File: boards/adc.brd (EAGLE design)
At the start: 49.6 x 25.6 mm, 42 parts, among them U1 ADS1194CPAG

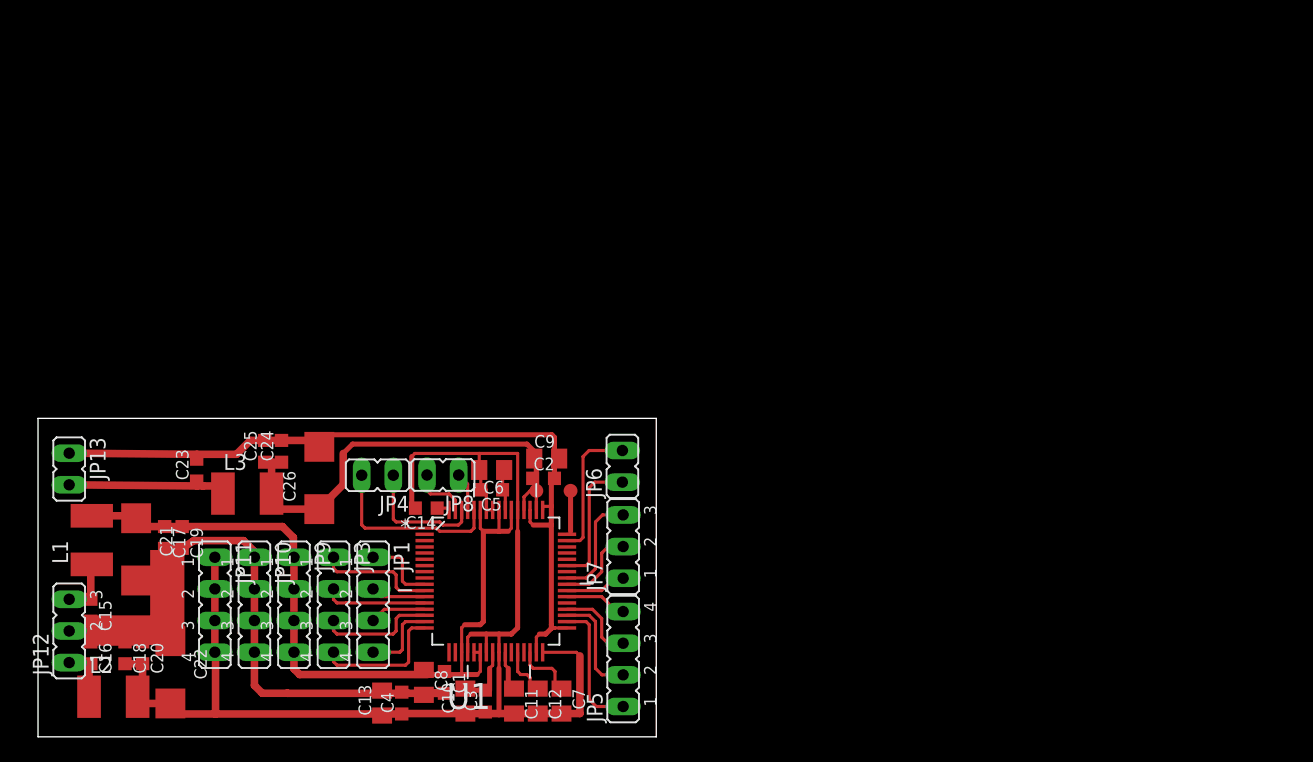
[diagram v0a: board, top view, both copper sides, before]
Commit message: put all the downloaded files into directories
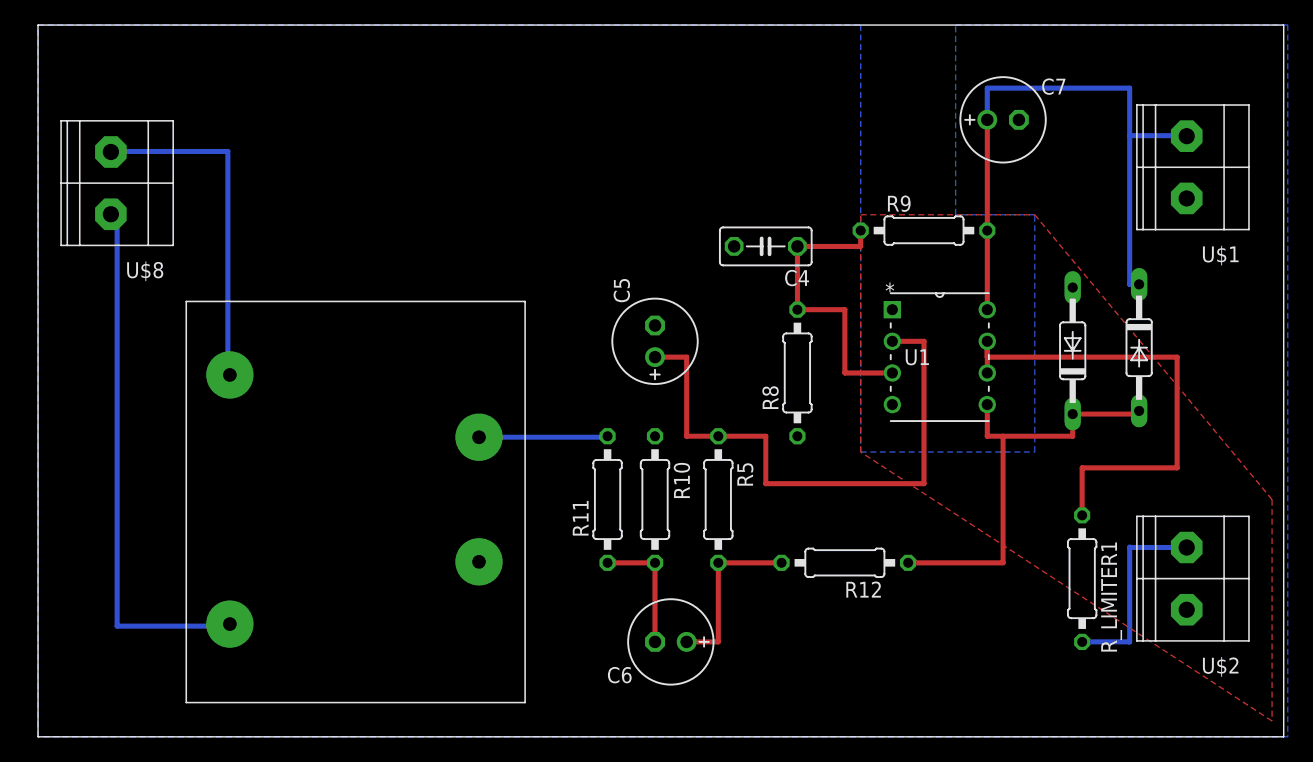
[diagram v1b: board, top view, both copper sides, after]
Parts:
- removed C1, C15, C16, C19, C2, C20, C23, C25, C3: 100n, rcl:C0603K
- removed C10, C12: 10u, rcl:C0805K
- removed C11, C13, C8, C9: 1u, rcl:C0805K
- removed C14, C17, C18, C24: 100p, rcl:C0603K
- removed C21, C22, C26: 47u, rcl:SMC_C
- removed JP1: AINneg, jumper:JP4
- removed JP10: AINgnd, jumper:JP4
- removed JP11: AINvss, jumper:JP4
- removed JP12: PWR1, jumper:JP2
- removed JP13: PWR2, jumper:JP1
- removed JP3: AINpos, jumper:JP4
- removed JP4: RL2, jumper:JP1
- removed JP5: CTRL2, jumper:JP4
- removed JP6: CTRL1, jumper:JP1
- removed JP7: CTRL2, jumper:JP2
- removed JP8: RL1, jumper:JP1
- removed JP9: AINvdd, jumper:JP4
- removed L1, L2, L3: 22u, rcl:L1812
- added R10, R11, R12, R5, R8, R9, R_LIMITER1: (no value), ee2parts:0207/10
- added U$1, U$2, U$8: CTB1500/2, eko-parts:CTB1500-2
- added U$5: (no value), Pauls_parts:4408
- added U$6, U$7: SD103A, Pauls_parts:D035-10
- C4: value 100n -> (none); device rcl:C0603K -> ee2parts:C050-030-075
- C5: value 100n -> (none); device rcl:C0603K -> ee2parts:E2,5-7---100UF
- C6, C7: value 1u -> (none); device rcl:C0805K -> ee2parts:E2,5-7---100UF
- U1: value ADS1194CPAG -> MCP602-E/P; device adc-ti:QFP50P1200X1200X120-64N -> MCP:DIP254P762X508-8P
- moved C7 58.6 mm to (77.5, 49.5), turned to 0 degrees
- moved C4 46.9 mm to (58.4, 39.4), turned to 180 degrees
- moved U1 41.9 mm to (76.2, 26.7)
- moved C6 19.9 mm to (50.8, 7.62)
- moved C5 17.7 mm to (49.5, 31.8), turned to 90 degrees
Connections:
- removed net +2V5: C1.1, C17.1, C19.1, C21.+, C8.1, JP9.1, JP9.2, JP9.3, JP9.4, L1.2, U1.19, U1.21, U1.22, U1.54, U1.56, U1.59
- removed net +2V5/1: C15.1, JP12.3, L1.1
- removed net +3V3: C2.1, C24.1, C25.1, C26.+, C9.1, L3.2, U1.48, U1.50, U1.52
- removed net +3V3/1: C23.1, JP13.2, L3.1
- removed net -2V5: C10.1, C11.2, C12.2, C13.1, C14.2, C18.2, C20.2, C22.-, C3.1, C4.1, C5.2, C6.2, C7.2, JP11.1, JP11.2, JP11.3, JP11.4, L2.2, U1.20, U1.23, U1.25, U1.32, U1.53, U1.57, U1.58
- removed net -2V5/1: C16.2, JP12.1, L2.1
- removed net AGND: C1.2, C13.2, C15.2, C16.1, C17.2, C18.1, C19.2, C20.1, C21.-, C22.+, C4.2, C8.2, JP10.1, JP10.2, JP10.3, JP10.4, JP12.2
- removed net DAISY_IN: JP7.3, U1.41
- removed net DIN: JP5.1, U1.34
- removed net DOUT: JP6.1, U1.43
- removed net N$11: JP3.1, U1.10
- removed net N$13: JP3.3, U1.14
- removed net N$14: JP3.2, U1.12
- removed net N$15: JP4.1, U1.62
- removed net N$16: JP4.2, U1.60
- removed net N$24: JP8.2, U1.63
- removed net N$3: C7.1, U1.30
- removed net N$4: C12.1, U1.28
- removed net N$5: C11.1, U1.26
- removed net N$6: JP1.4, U1.15
- removed net N$7: C14.1, U1.64
- removed net N$8: JP1.3, U1.13
- removed net N$9: JP1.2, U1.11
- removed net SCLK: JP7.2, U1.40
- removed net START: JP5.4, U1.38
- removed net ~CS: JP7.1, U1.39
- removed net ~DRDY: JP6.2, U1.47
- removed net ~PWDN: JP5.2, U1.35
- removed net ~RESET: JP5.3, U1.36
- new net N$18: R11.2, U$5.PIN7
- new net N$21: C6.+, R12.2, R5.2
- new net V+: C7.+, R9.2, U$1.P$2, U$6.C, U1.8
- new net V_IN1: U$5.PIN5, U$8.P$2
- new net V_IN2: U$5.PIN1, U$8.P$1
- new net V_OUT: R_LIMITER1.2, U$2.P$2
- net GND: now also C4.2, C5.-, C7.-, R10.1, R8.1, U$2.P$1, U$5.PIN9, U$7.A, U1.4; no longer C2.2, C23.2, C24.2, C25.2, C26.-, C9.2, JP13.1, U1.31, U1.33, U1.49, U1.51
- net N$1: now also R_LIMITER1.1, U1.6, U1.7; no longer C10.2, C3.2, U1.24
- net N$10: now also C4.1, R8.2, R9.1, U1.3; no longer JP1.1, U1.9
- net N$12: now also R12.1, U$6.A, U$7.C, U1.5; no longer JP3.4, U1.16
- net N$17: now also C6.-, R10.2, R11.1; no longer JP8.1, U1.61
- net N$2: now also C5.+, R5.1, U1.1, U1.2; no longer C5.1, C6.1, U1.55
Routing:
- net -2V5: track 109.1 -> 0.00 mm
- net +2V5: track 66.4 -> 0.00 mm
- net GND: track 65.5 -> 0.00 mm
- net AGND: track 56.6 -> 0.00 mm
- net V+: track 0.00 -> 50.3 mm
- net V_IN2: track 0.00 -> 42.8 mm
- net N$2: track 3.55 -> 45.7 mm
- net +3V3: track 41.2 -> 0.00 mm
- net N$1: track 5.12 -> 39.4 mm
- net V_IN1: track 0.00 -> 27.5 mm
- net N$12: track 10.9 -> 34.5 mm
- net N$10: track 6.06 -> 24.1 mm
- net V_OUT: track 0.00 -> 16.0 mm
- net N$16: track 14.8 -> 0.00 mm
- net N$21: track 0.00 -> 14.0 mm
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- added copper zone on layer 1, net GND
- added copper zone on layer 16, net GND
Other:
- board size 49.6 x 25.6 mm -> 100 x 57.1 mm
- board text removed: "+2V5"
- board text removed: "+3V3"
- board text removed: "-2V5"
- board text removed: "AGND"
- board text removed: "DAISY"
- board text removed: "DGND"
- board text removed: "DIN"
- board text removed: "DOUT"
- board text removed: "IN+"
- board text removed: "IN-"
- board text removed: "MindSpy.org"
- board text removed: "SCLK"
- board text removed: "START"
- board text removed: "adc board ver. 0.1"
- board text removed: "~CS"
- board text removed: "~DRDY"
- board text removed: "~PWRDN"
- board text removed: "~RESET"
